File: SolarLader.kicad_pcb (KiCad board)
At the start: 2 copper layers, 26 x 18 mm, 26 parts, among them J1 Conn_01x02, J2 UKDBBTAAA, J3 Conn_01x02, Q1 Q_PMOS_GSD, U1 BQ25185DLHR

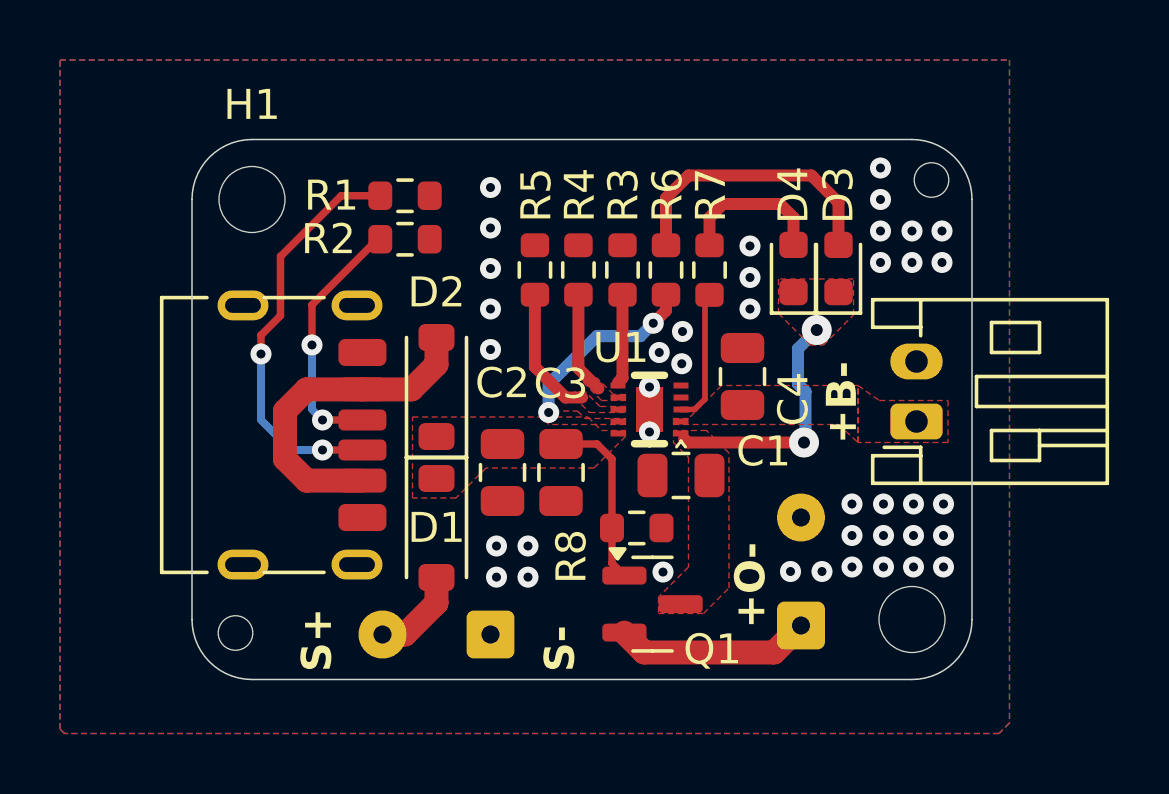
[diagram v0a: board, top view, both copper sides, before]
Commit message: ReleaseCandidate1
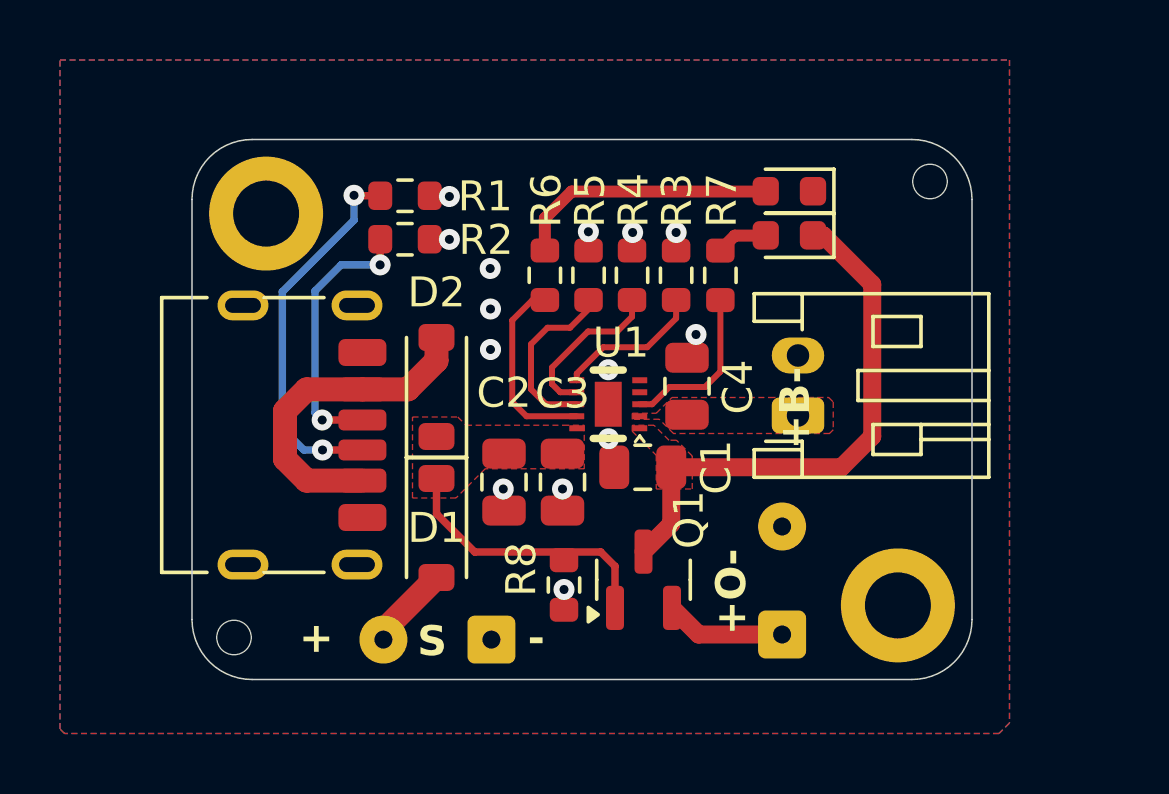
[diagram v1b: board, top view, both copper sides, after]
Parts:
- removed H1, H2: MountingHole, MountingHole:MountingHole_2.2mm_M2
- added H3: MountingHole_Pad, MountingHole:MountingHole_2.2mm_M2_DIN965_Pad, F.Cu at (134.0, 65.1)
- added H4: MountingHole_Pad, MountingHole:MountingHole_2.2mm_M2_DIN965_Pad, F.Cu at (155.0, 78.1)
- R4: value 13k -> 5k
- R5: value 600 -> 1k
- moved R6 4.04 mm to (143.3, 67.1)
- moved BT1 3.96 mm to (151.7, 71.8)
- moved R8 3.08 mm to (143.9, 77.5), turned to -90 degrees
- moved D3 3.05 mm to (151.4, 64.3), turned to 180 degrees
- moved C4 1.88 mm to (148.0, 70.8)
- moved R3 1.80 mm to (147.6, 67.1)
- moved R4 1.80 mm to (146.2, 67.1)
- moved R5 1.80 mm to (144.7, 67.1)
- moved U1 1.39 mm to (145.4, 71.4)
- moved C1 1.30 mm to (146.5, 73.5)
- moved D4 1.11 mm to (151.4, 65.8), turned to 180 degrees
- moved Q1 0.87 mm to (146.6, 77.3), turned to 90 degrees
- moved J3 0.70 mm to (151.2, 79.1)
- moved R7 0.40 mm to (149.1, 67.1)
- moved C2 0.32 mm to (141.9, 74.0)
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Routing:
- net VSYS: track 8.18 -> 18.0 mm, vias 2 -> 0
- net Net-(D4-A): track 5.01 -> 1.73 mm
- net VIN: track 5.97 -> 9.24 mm
- net Net-(J3-Pin_1): track 6.53 -> 4.04 mm
- net /VSET: track 3.40 -> 5.42 mm
- net /TS/MR: track 2.99 -> 4.91 mm
- net /ISET: track 4.40 -> 5.94 mm
- net Net-(J2-CC2): track 13.7 -> 12.6 mm
- net /STAT2: track 4.48 -> 5.52 mm
- net Net-(J2-CC1): track 8.49 -> 9.13 mm
- net Net-(D3-A): track 9.42 -> 8.81 mm
- net GND: track 0.00 -> 0.15 mm, vias 40 -> 14
- net /STAT1: track 6.39 -> 6.44 mm, vias 2 -> 0
- removed copper zone on F.Cu, net /ISET
- removed copper zone on F.Cu, net /STAT1
- removed copper zone on F.Cu, net /VSET
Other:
- board text added: "+"
- board text added: "-"
- board text added: "S"
- board text removed: "S+"
- board text removed: "S-"
